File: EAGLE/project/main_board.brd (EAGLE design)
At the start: 85 x 56 mm, 14 parts

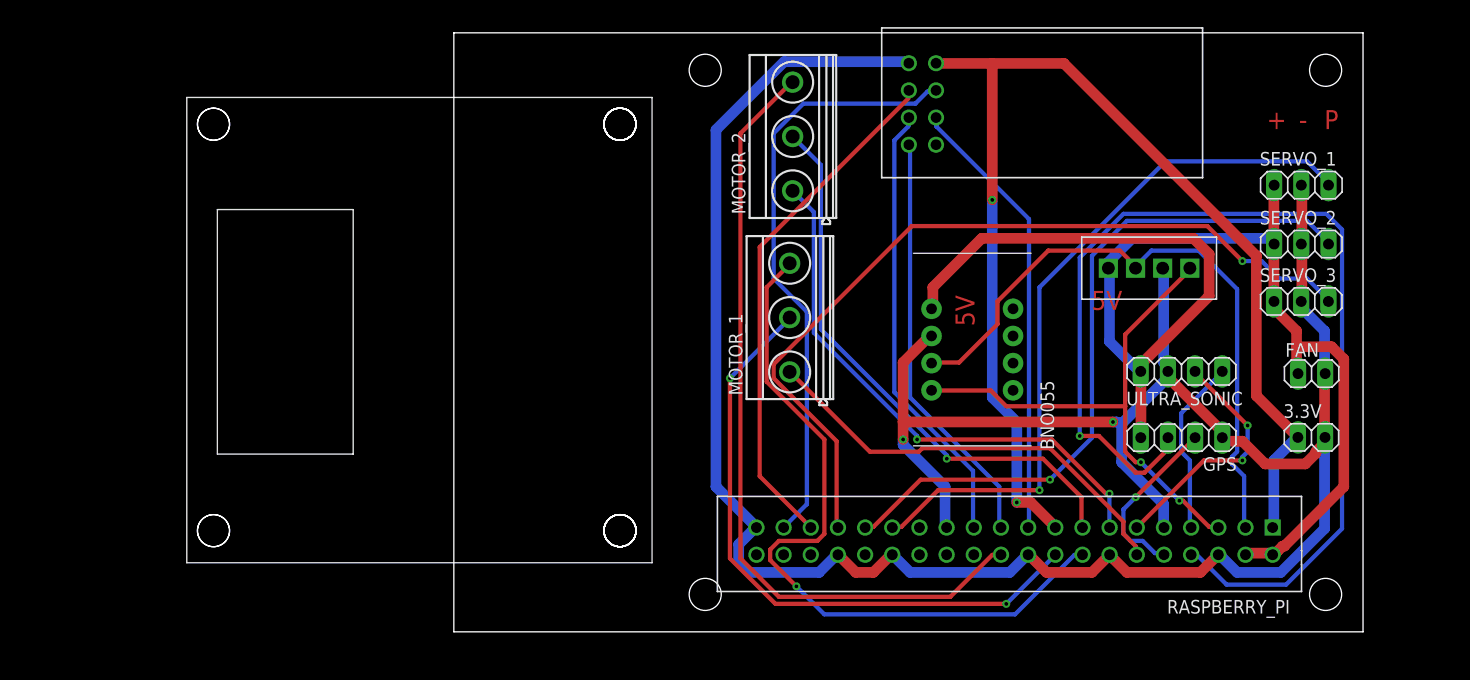
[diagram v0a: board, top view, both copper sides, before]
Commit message: update main board
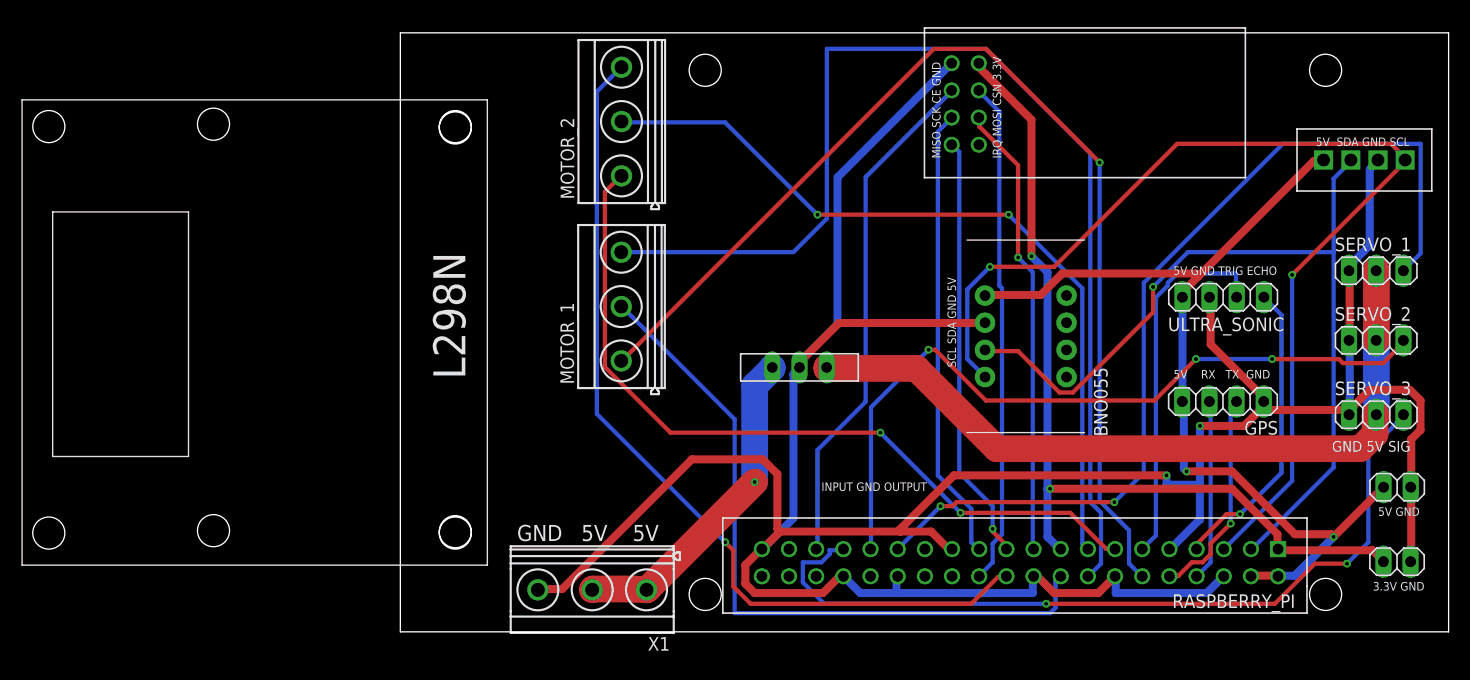
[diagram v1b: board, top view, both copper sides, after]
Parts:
- added LXDC1: LXDC55, LXDC55:LXDC55
- added X1: MKDSN1,5/3-5,08, con-phoenix-508:MKDSN1,5/3-5,08
- moved U$1 22.5 mm to (0.13, 44.1)
- moved MOTOR_2 16.1 mm to (-69.3, 50.3)
- moved MOTOR_1 15.8 mm to (-69.3, 33.0)
- moved L298N1 15.4 mm to (-81.9, 6.24)
- moved 3.3V 14.1 mm to (3.18, 6.56)
- moved FAN 13.3 mm to (3.19, 13.5)
- moved SERVO_3 12.7 mm to (1.24, 20.3)
- moved SERVO_2 11.4 mm to (1.23, 27.3)
- moved SERVO_1 10.6 mm to (1.23, 33.8)
- moved ULTRA_SONIC 7.95 mm to (-13.1, 31.3)
- moved BNO055 5.15 mm to (-31.5, 27.6)
- moved GPS 5.14 mm to (-13.1, 21.5)
- moved NRF24L1 4.00 mm to (-41.0, 43.0)
- moved RASPBERRY_PI 2.08 mm to (-42.1, 31.0)
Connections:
- net N$1 renamed CE
- net N$3 renamed SCK
- net N$4 renamed MOSI
- net N$5 renamed MISO
- net ULTRA_SONIC_1 renamed ECHO
- net ULTRA_SONIC_2 renamed TRIG
- removed net N$2: NRF24L1.CSN, RASPBERRY_PI.37
- new net 5V_LXDC55: LXDC1.OUTPUT, SERVO_1.2, SERVO_2.2, SERVO_3.2
- new net BATTERY+: LXDC1.INPUT, X1.1, X1.2
- new net CSN: NRF24L1.CSN, RASPBERRY_PI.24
- net 5V: no longer SERVO_1.1, SERVO_2.1, SERVO_3.1
- net GND: now also LXDC1.GND, SERVO_1.1, SERVO_2.1, SERVO_3.1, X1.3; no longer SERVO_1.2, SERVO_2.2, SERVO_3.2
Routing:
- net RX: track 100.6 -> 17.0 mm, vias 1 -> 0
- net 5V_LXDC55: track 0.00 -> 70.4 mm
- net ENA: track 40.9 -> 101.6 mm, vias 0 -> 1
- net N$2: track 55.9 -> 0.00 mm
- net GND: track 249.8 -> 302.5 mm
- net BNO055_SCL: track 50.0 -> 99.7 mm
- net CSN: track 0.00 -> 47.2 mm
- net 5V: track 126.0 -> 88.3 mm, vias 0 -> 2
- net IN2: track 68.7 -> 105.6 mm, vias 1 -> 0
- net BATTERY+: track 0.00 -> 30.8 mm, vias 0 -> 1
- net 3.3V: track 112.0 -> 83.7 mm
- net IN3: track 51.3 -> 73.3 mm
- net IN4: track 53.1 -> 74.1 mm, vias 1 -> 2
- net BNO055_SDA: track 60.5 -> 81.4 mm, vias 0 -> 1
- net PWM_SERVO_1: track 67.2 -> 87.5 mm, vias 1 -> 2
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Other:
- board size 85 x 56 mm -> 98 x 56 mm
- board text added: "3.3V GND"
- board text added: "5V GND"
- board text added: "5V GND TRIG ECHO"
- board text added: "5V RX TX GND"
- board text added: "5V SDA GND SCL"
- board text added: "GND 5V 5V"
- board text added: "GND 5V SIG"
- board text added: "INPUT GND OUTPUT"
- board text added: "IRQ MOSI CSN 3.3V"
- board text added: "L298N"
- board text added: "MISO SCK CE GND"
- board text added: "SCL SDA GND 5V"
- board text removed: "+"
- board text removed: "-"
- board text removed: "5V"
- board text removed: "P"
